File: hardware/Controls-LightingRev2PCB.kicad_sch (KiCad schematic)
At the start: 39 parts, among them IC3 TLV70130DBVR, J1 MX150_02x08_RightAngle, J3 53307-2471, Q2 IRLML0030, Q3 IRLML0030, U1 TLV2371DBV, U2 INA241A5xD, U3 INA241A5xD, U4 INA241A5xD, U5 SN74LV1T34DBV, U8 TLV2371DBV, U9 TLV2371DBV

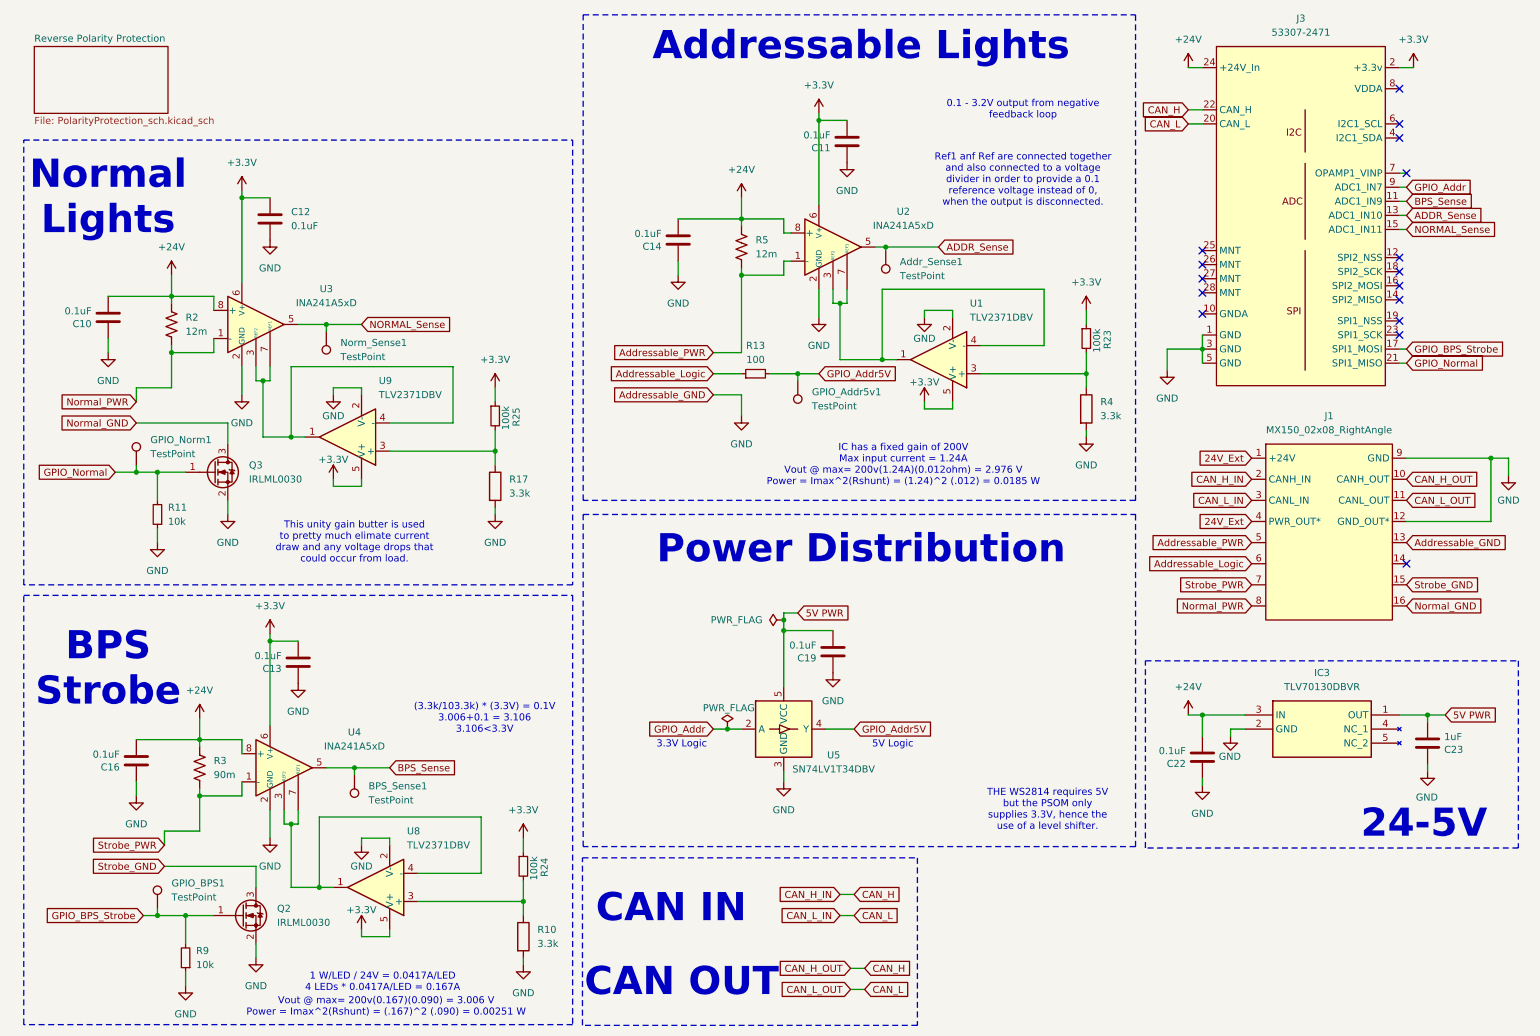
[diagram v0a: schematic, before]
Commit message: BOM
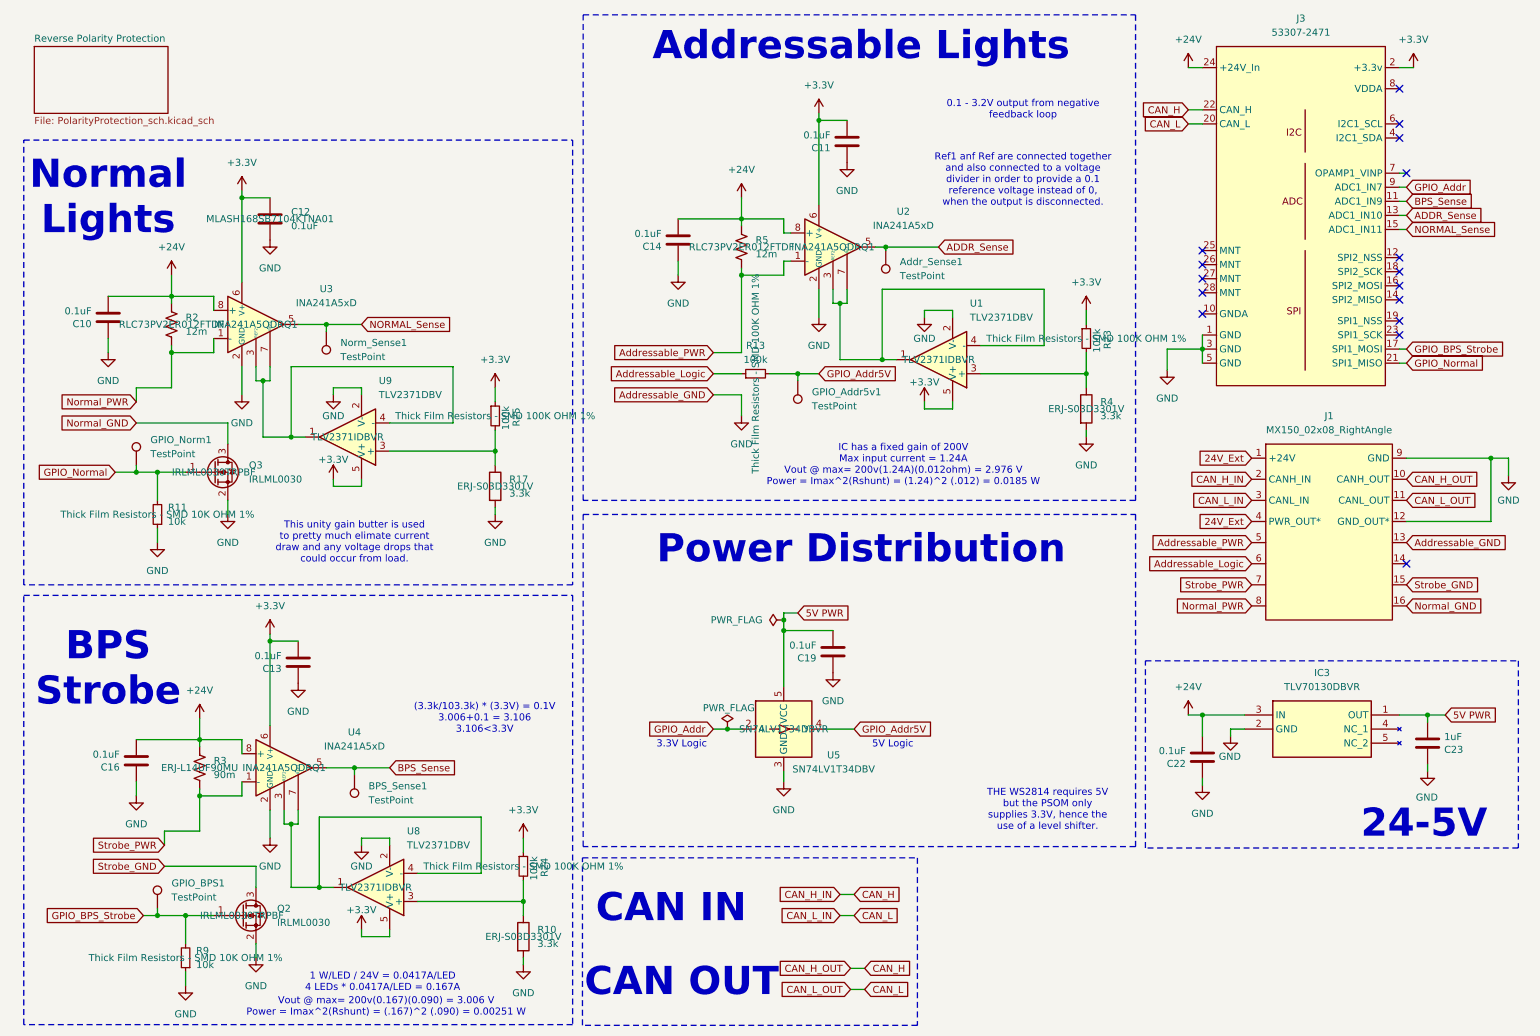
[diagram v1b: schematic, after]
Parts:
- C12: P/N (none) -> MLASH168SB7104KTNA01
- C22: P/N MLASU168SB5105KTNA01 -> MLASH168SB7104KTNA01
- Q2, Q3: P/N (none) -> IRLML0030TRPBF
- R10, R17, R4: P/N (none) -> ERJ-S03D3301V
- R11, R9: P/N CRCW080510K0FKEAC -> CRCW060310K0FKEI
- R13: value 100 -> 100k; P/N SDR10EZPF1001 -> CRCW0603100KFKEE
- R2, R5: P/N (none) -> RLC73PV2ER012FTDF
- R23, R24, R25: P/N CRCW0805100KFKEAC -> CRCW0603100KFKEE
- R3: P/N (none) -> ERJ-L14UF90MU
- U1, U8, U9: P/N (none) -> TLV2371IDBVR
- U2, U3, U4: P/N (none) -> INA241A5QDRQ1
- U5: P/N (none) -> SN74LV1T34DBVR
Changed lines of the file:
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@@
 			)
 		)
-		(property "Description" ""
+		(property "Description" "Thick Film Resistors - SMD 100K OHM 1%"
 			(at 104.14 167.64 0)
 			(effects
@@
 			)
 		)
-		(property "P/N" "CRCW0805100KFKEAC"
+		(property "P/N" "CRCW0603100KFKEE"
 			(at 104.14 167.64 0)
 			(effects
@@
 			)
 		)
-		(property "Description" "Unpolarized capacitor"
+		(property "Description" "Multilayer Ceramic Capacitors MLCC - SMD/SMT 100V 0.1uF X7R 0603 10% Medical"
 			(at 132.08 54.61 0)
 			(effects
@@
 			)
 		)
-		(property "Description" "Unpolarized capacitor"
+		(property "Description" "Multilayer Ceramic Capacitors MLCC - SMD/SMT 100V 0.1uF X7R 0603 10% Medical"
 			(at 29.21 68.58 0)
 			(effects
@@
 			)
 		)
-		(property "Description" "Resistor"
+		(property "Description" "Thick Film Resistors - SMD 0603 0.5% 3.3kOhm Anti-Sulfur AEC-Q200"
 			(at 205.74 85.09 0)
 			(effects
@@
 			)
 		)
+		(property "P/N" "ERJ-S03D3301V"
+			(at 205.74 85.09 0)
+			(effects
+				(font
+					(size 1.27 1.27)
+				)
+			)
+		)
 		(pin "2"
 		)
@@
 			)
 		)
-		(property "Description" "Rail-to-Rail Input/Output Operational Amplifier, SOT-23-5"
+		(property "Description" "Operational Amplifiers - Op Amps 550uA/Ch 3MHz R/R Op A 595-TLV2371IDBVT"
 			(at 179.07 76.2 0)
 			(effects
@@
 			)
 		)
+		(property "P/N" "TLV2371IDBVR"
+			(at 179.07 76.2 0)
+			(effects
+				(font
+					(size 1.27 1.27)
+				)
+			)
+		)
 		(pin "5"
 		)
@@
 			)
 		)
-		(property "Description" ""
+		(property "Description" "Thick Film Resistors - SMD 10K OHM 1%"
 			(at 43.18 184.15 0)
 			(effects
@@
 			)
 		)
-		(property "P/N" "CRCW080510K0FKEAC"
+		(property "P/N" "CRCW060310K0FKEI "
 			(at 43.18 184.15 0)
 			(effects
@@
 			)
 		)
-		(property "Description" ""
+		(property "Description" "Thick Film Resistors - SMD 10K OHM 1%"
 			(at 38.1 104.14 0)
 			(effects
@@
 			)
 		)
-		(property "P/N" "CRCW080510K0FKEAC"
+		(property "P/N" "CRCW060310K0FKEI "
 			(at 38.1 104.14 0)
 			(effects
@@
 			)
 		)
-		(property "Description" "Unpolarized capacitor"
+		(property "Description" "Multilayer Ceramic Capacitors MLCC - SMD/SMT 100V 0.1uF X7R 0603 10% Medical"
 			(at 162.56 36.83 0)
 			(effects
@@
 			)
 		)
-		(property "Description" "Unpolarized capacitor"
+		(property "Description" "Multilayer Ceramic Capacitors MLCC - SMD/SMT 100V 0.1uF X7R 0603 10% Medical"
 			(at 226.695 147.955 0)
 			(effects
@@
 			)
 		)
-		(property "P/N" "MLASU168SB5105KTNA01"
+		(property "P/N" "MLASH168SB7104KTNA01"
 			(at 226.695 147.955 0)
 			(effects
@@
 			)
 		)
-		(property "Description" "Unpolarized capacitor"
+		(property "Description" "Multilayer Ceramic Capacitors MLCC - SMD/SMT 50V 1uF X5R 0603 10%"
 			(at 267.335 145.415 0)
 			(effects
@@
 			)
 		)
-		(property "Description" "Resistor, US symbol"
+		(property "Description" "Current Sense Resistors - SMD 1210 90mOhm 1% Curr Sense AEC-Q200"
 			(at 45.72 149.86 0)
 			(effects
@@
 			)
 		)
+		(property "P/N" "ERJ-L14UF90MU"
+			(at 45.72 149.86 0)
+			(effects
+				(font
+					(size 1.27 1.27)
+				)
+			)
+		)
 		(pin "1"
 		)
@@
 			)
 		)
-		(property "Value" "100"
+		(property "Value" "100k"
 			(at 146.05 76.2 90)
 			(effects
@@
 			)
 		)
-		(property "Description" ""
+		(property "Description" "Thick Film Resistors - SMD 100K OHM 1%"
 			(at 146.05 78.74 0)
 			(effects
@@
 			)
 		)
-		(property "P/N" "SDR10EZPF1001"
+		(property "P/N" "CRCW0603100KFKEE"
 			(at 146.05 78.74 0)
 			(effects
@@
 			)
 		)
-		(property "Description" "Resistor"
+		(property "Description" "Thick Film Resistors - SMD 0603 0.5% 3.3kOhm Anti-Sulfur AEC-Q200"
 			(at 99.06 99.06 0)
 			(effects
@@
 			)
 		)
+		(property "P/N" "ERJ-S03D3301V"
+			(at 99.06 99.06 0)
+			(effects
+				(font
+					(size 1.27 1.27)
+				)
+			)
+		)
 		(pin "2"
 		)
@@
 			)
 		)
-		(property "Description" "5.3A Id, 30V Vds, 27mOhm Rds, N-Channel HEXFET Power MOSFET, SOT-23"
+		(property "Description" "MOSFETs MOSFT 30V 5.2A 28mOhm 3.6nC Qg"
 			(at 48.26 96.52 0)
 			(effects
@@
 			)
 		)
+		(property "P/N" "IRLML0030TRPBF"
+			(at 48.26 96.52 0)
+			(effects
+				(font
+					(size 1.27 1.27)
+				)
+			)
+		)
 		(pin "1"
 		)
@@
 			)
 		)
-		(property "Description" ""
+		(property "Description" "Thick Film Resistors - SMD 100K OHM 1%"
 			(at 99.06 86.36 0)
 			(effects
@@
 			)
 		)
-		(property "P/N" "CRCW0805100KFKEAC"
+		(property "P/N" "CRCW0603100KFKEE"
 			(at 99.06 86.36 0)
 			(effects
@@
 			)
 		)
-		(property "Description" "Resistor, US symbol"
+		(property "Description" "Current Sense Resistors - SMD RLC73PV 2E R012 1% 1K RL"
 			(at 40.64 69.85 0)
 			(effects
@@
 			)
 		)
+		(property "P/N" "RLC73PV2ER012FTDF"
+			(at 40.64 69.85 0)
+			(effects
+				(font
+					(size 1.27 1.27)
+				)
+			)
+		)
 		(pin "1"
 		)
@@
 			)
 		)
-		(property "Description" "Unpolarized capacitor"
+		(property "Description" "Multilayer Ceramic Capacitors MLCC - SMD/SMT 100V 0.1uF X7R 0603 10% Medical"
 			(at 34.29 148.59 0)
 			(effects
@@
 			)
 		)
-		(property "Description" "Resistor, US symbol"
+		(property "Description" "Current Sense Resistors - SMD RLC73PV 2E R012 1% 1K RL"
 			(at 143.51 55.88 0)
 			(effects
@@
 			)
 		)
+		(property "P/N" "RLC73PV2ER012FTDF"
+			(at 143.51 55.88 0)
+			(effects
+				(font
+					(size 1.27 1.27)
+				)
+			)
+		)
 		(pin "1"
 		)
@@
 			)
 		)
-		(property "Description" ""
+		(property "Description" "Thick Film Resistors - SMD 100K OHM 1%"
 			(at 205.74 72.39 0)
 			(effects
@@
 			)
 		)
-		(property "P/N" "CRCW0805100KFKEAC"
+		(property "P/N" "CRCW0603100KFKEE"
 			(at 205.74 72.39 0)
 			(effects
@@
 			)
 		)
-		(property "Description" "Unpolarized capacitor"
+		(property "Description" "Multilayer Ceramic Capacitors MLCC - SMD/SMT 100V 0.1uF X7R 0603 10% Medical"
 			(at 160.02 128.905 0)
 			(effects
@@
 			)
 		)
-		(property "Description" "Rail-to-Rail Input/Output Operational Amplifier, SOT-23-5"
+		(property "Description" "Operational Amplifiers - Op Amps 550uA/Ch 3MHz R/R Op A 595-TLV2371IDBVT"
 			(at 77.47 171.45 0)
 			(effects
@@
 			)
 		)
+		(property "P/N" "TLV2371IDBVR"
+			(at 77.47 171.45 0)
+			(effects
+				(font
+					(size 1.27 1.27)
+				)
+			)
+		)
 		(pin "5"
 		)
@@
 			)
 		)
-		(property "Description" "High- and Low-Side, Bidirectional, Zero-Drift, Current-Sense Amplifier With Enhanced PWM Rejection, 200V/V, ±0.01% Gain Accuracy, ±10 μV Offset Voltage, SOIC-8"
+		(property "Description" "Current Sense Amplifiers AEC-Q100 -4V to 110 V bidirectional ultr"
 			(at 160.02 55.88 0)
 			(effects
@@
 			)
 		)
+		(property "P/N" "INA241A5QDRQ1"
+			(at 160.02 55.88 0)
+			(effects
+				(font
+					(size 1.27 1.27)
+				)
+			)
+		)
 		(pin "1"
 		)
@@
 			)
 		)
-		(property "Description" "Unpolarized capacitor"
+		(property "Description" "Multilayer Ceramic Capacitors MLCC - SMD/SMT 100V 0.1uF X7R 0603 10% Medical"
 			(at 63.5 130.81 0)
 			(effects
@@
 			)
 		)
-		(property "Description" "Single Power Supply, Single Buffer GATE, CMOS Logic, Level Shifter, SOT-23-5"
+		(property "Description" "Translation - Voltage Levels SGL Pwr Spply Buffer GATE CMOS"
 			(at 151.13 142.875 0)
 			(effects
@@
 			)
 		)
+		(property "P/N" "SN74LV1T34DBVR"
+			(at 151.13 142.875 0)
+			(effects
+				(font
+					(size 1.27 1.27)
+				)
+			)
+		)
 		(pin "2"
 		)
@@
 			)
 		)
-		(property "Description" "Unpolarized capacitor"
+		(property "Description" "Multilayer Ceramic Capacitors MLCC - SMD/SMT 100V 0.1uF X7R 0603 10% Medical"
 			(at 58.42 50.8 0)
 			(effects
@@
 			)
 		)
+		(property "P/N" "MLASH168SB7104KTNA01"
+			(at 58.42 50.8 0)
+			(effects
+				(font
+					(size 1.27 1.27)
+				)
+			)
+		)
 		(pin "1"
 		)
@@
 			)
 		)
-		(property "Description" "High- and Low-Side, Bidirectional, Zero-Drift, Current-Sense Amplifier With Enhanced PWM Rejection, 200V/V, ±0.01% Gain Accuracy, ±10 μV Offset Voltage, SOIC-8"
+		(property "Description" "Current Sense Amplifiers AEC-Q100 -4V to 110 V bidirectional ultr"
 			(at 55.88 69.85 0)
 			(effects
@@
 			)
 		)
+		(property "P/N" "INA241A5QDRQ1"
+			(at 55.88 69.85 0)
+			(effects
+				(font
+					(size 1.27 1.27)
+				)
+			)
+		)
 		(pin "1"
 		)
@@
 			)
 		)
-		(property "Description" "High- and Low-Side, Bidirectional, Zero-Drift, Current-Sense Amplifier With Enhanced PWM Rejection, 200V/V, ±0.01% Gain Accuracy, ±10 μV Offset Voltage, SOIC-8"
+		(property "Description" "Current Sense Amplifiers AEC-Q100 -4V to 110 V bidirectional ultr"
 			(at 60.96 149.86 0)
 			(effects
@@
 			)
 		)
+		(property "P/N" "INA241A5QDRQ1"
+			(at 60.96 149.86 0)
+			(effects
+				(font
+					(size 1.27 1.27)
+				)
+			)
+		)
 		(pin "1"
 		)
@@
 			)
 		)
-		(property "Description" "Rail-to-Rail Input/Output Operational Amplifier, SOT-23-5"
+		(property "Description" "Operational Amplifiers - Op Amps 550uA/Ch 3MHz R/R Op A 595-TLV2371IDBVT"
 			(at 72.39 90.17 0)
 			(effects
@@
 			)
 		)
+		(property "P/N" "TLV2371IDBVR"
+			(at 72.39 90.17 0)
+			(effects
+				(font
+					(size 1.27 1.27)
+				)
+			)
+		)
 		(pin "5"
 		)
@@
 			)
 		)
-		(property "Description" "5.3A Id, 30V Vds, 27mOhm Rds, N-Channel HEXFET Power MOSFET, SOT-23"
+		(property "Description" "MOSFETs MOSFT 30V 5.2A 28mOhm 3.6nC Qg"
 			(at 53.34 176.53 0)
 			(effects
@@
 			)
 		)
+		(property "P/N" "IRLML0030TRPBF"
+			(at 53.34 176.53 0)
+			(effects
+				(font
+					(size 1.27 1.27)
+				)
+			)
+		)
 		(pin "1"
 		)
@@
 			)
 		)
-		(property "Description" "Resistor"
+		(property "Description" "Thick Film Resistors - SMD 0603 0.5% 3.3kOhm Anti-Sulfur AEC-Q200"
 			(at 104.14 180.34 0)
 			(effects
@@
 			)
 		)
+		(property "P/N" "ERJ-S03D3301V"
+			(at 104.14 180.34 0)
+			(effects
+				(font
+					(size 1.27 1.27)
+				)
+			)
+		)

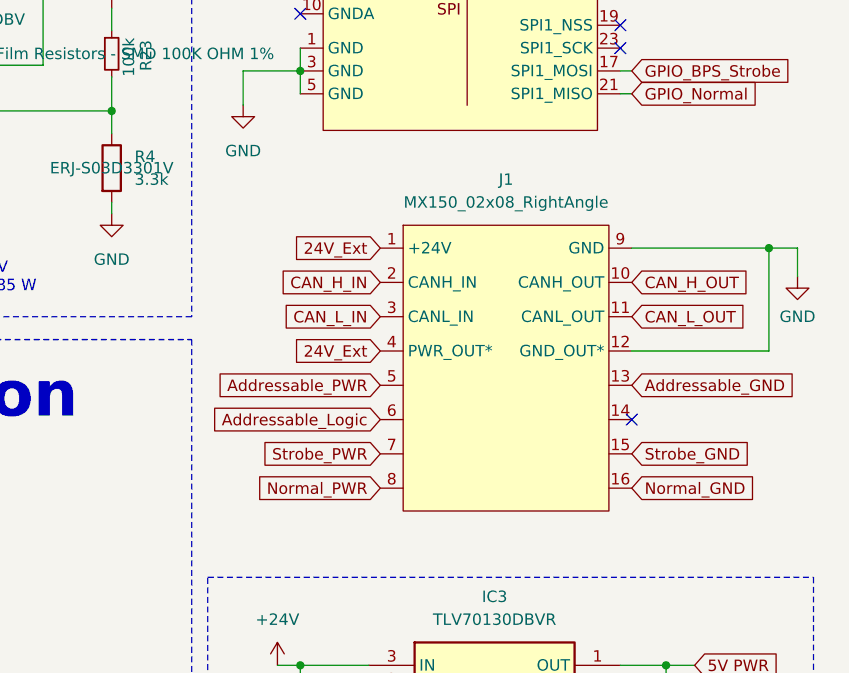
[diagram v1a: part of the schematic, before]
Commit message: RevA
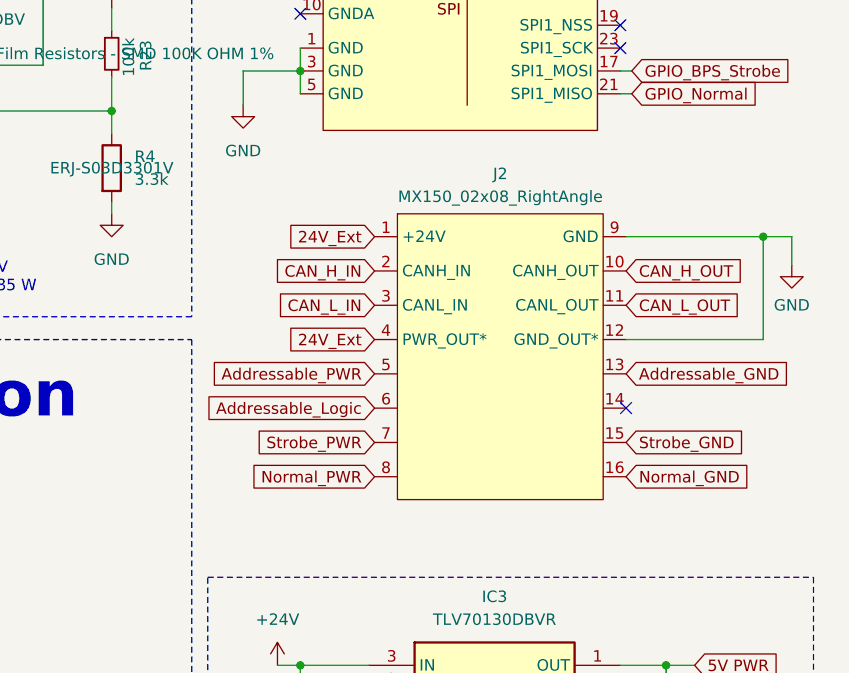
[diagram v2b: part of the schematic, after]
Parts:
- removed J1: MX150_02x08_RightAngle, UTSVT_Connectors:CONN_SD-75900-001_2X08_MOL, symbol UTSVT-Connectors:MX150_02x08_RightAngle
- added J2: MX150_02x08_RightAngle, UTSVT_Connectors:MX150_02x08_RightAngle, symbol UTSVT-Connectors:MX150_02x08_RightAngle
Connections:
- net 24V_Ext: now also J2.1 (+24V), J2.4 (PWR_OUT*)
- net Addressable_Logic: now also J2.6
- net Addressable_PWR: now also J2.5
- net CAN_H: now also J2.10 (CANH_OUT), J2.2 (CANH_IN)
- net CAN_L: now also J2.11 (CANL_OUT), J2.3 (CANL_IN)
- net GND: now also J2.12 (GND_OUT*), J2.13, J2.9 (GND)
- net Normal_GND: now also J2.16
- net Normal_PWR: now also J2.8
- net Strobe_GND: now also J2.15
- net Strobe_PWR: now also J2.7
